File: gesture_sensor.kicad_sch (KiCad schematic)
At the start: 13 parts, among them U4 LM385

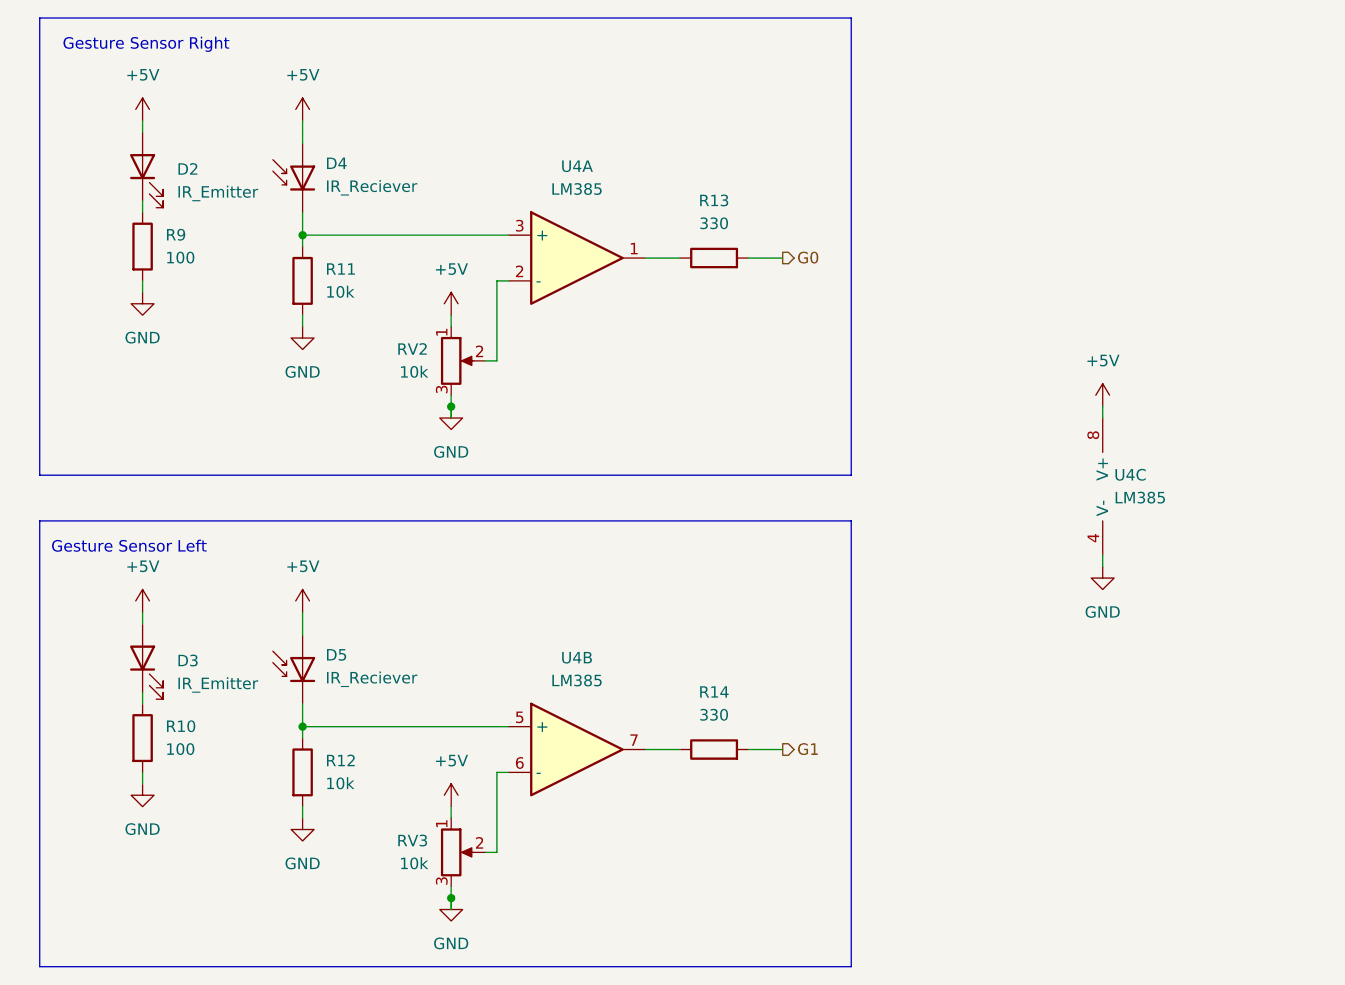
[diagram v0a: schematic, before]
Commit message: Finalized Schematic
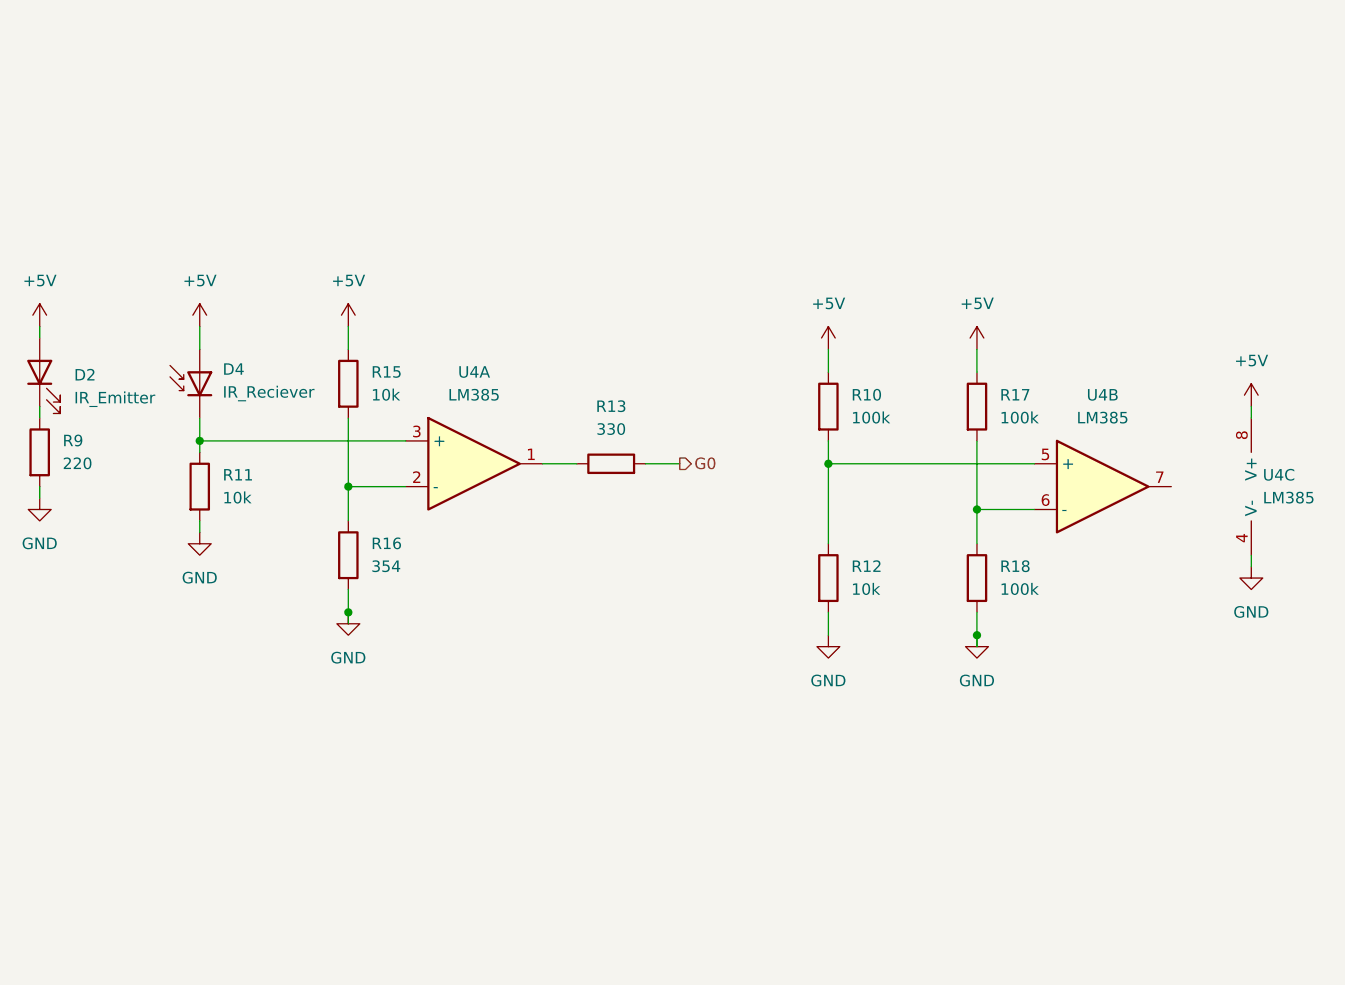
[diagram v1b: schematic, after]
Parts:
- removed D3: IR_Emitter, symbol Device:LED
- removed D5: IR_Reciever, symbol Device:D_Photo
- removed R14: 330, symbol Device:R
- removed RV2, RV3: 10k, symbol Device:R_Potentiometer
- added R15: 10k, symbol Device:R
- added R16: 354, symbol Device:R
- added R17, R18: 100k, symbol Device:R
- R10: value 100 -> 100k
- R9: value 100 -> 220
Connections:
- net +5V: now also R10.1, R15.1, R17.1
- net GND: now also R16.2, R18.2; no longer R10.2
- net at R12.1, U4.5 (+): now also R10.2
- net at U4.6 (-): now also R17.2, R18.1
- net at U4.2 (-): now also R15.2, R16.1
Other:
- note removed: "Gesture Sensor Left"
- note removed: "Gesture Sensor Right"
- moved on the sheet: D2, D4, R11, R12, R13, R9, U4A, U4B, U4C
